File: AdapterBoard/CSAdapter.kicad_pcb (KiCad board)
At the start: 2 copper layers, 10.4 x 18 mm, 3 parts, among them J1 Conn_01x04, J2 Conn_01x06, SW1 CHS-01

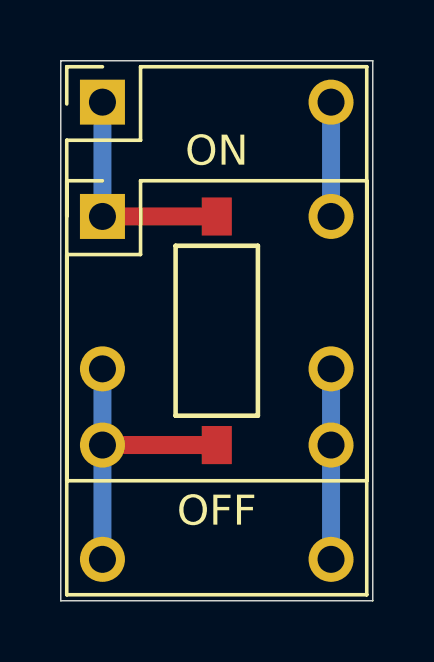
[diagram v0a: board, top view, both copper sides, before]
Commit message: Design rules and gerber files
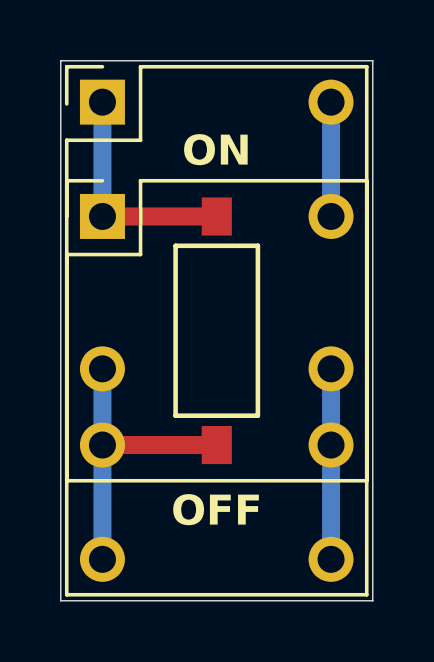
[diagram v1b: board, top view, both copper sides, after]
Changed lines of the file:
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@@
 	)
 	(setup
+		(stackup
+			(layer "F.SilkS"
+				(type "Top Silk Screen")
+			)
+			(layer "F.Paste"
+				(type "Top Solder Paste")
+			)
+			(layer "F.Mask"
+				(type "Top Solder Mask")
+				(thickness 0.01)
+			)
+			(layer "F.Cu"
+				(type "copper")
+				(thickness 0.035)
+			)
+			(layer "dielectric 1"
+				(type "core")
+				(thickness 1.51)
+				(material "FR4")
+				(epsilon_r 4.5)
+				(loss_tangent 0.02)
+			)
+			(layer "B.Cu"
+				(type "copper")
+				(thickness 0.035)
+			)
+			(layer "B.Mask"
+				(type "Bottom Solder Mask")
+				(thickness 0.01)
+			)
+			(layer "B.Paste"
+				(type "Bottom Solder Paste")
+			)
+			(layer "B.SilkS"
+				(type "Bottom Silk Screen")
+			)
+			(copper_finish "None")
+			(dielectric_constraints no)
+		)
 		(pad_to_mask_clearance 0)
 		(allow_soldermask_bridges_in_footprints no)
@@
 			(plot_on_all_layers_selection 0x0000000_00000000)
 			(disableapertmacros no)
-			(usegerberextensions no)
+			(usegerberextensions yes)
 			(usegerberattributes yes)
 			(usegerberadvancedattributes yes)
-			(creategerberjobfile yes)
+			(creategerberjobfile no)
 			(dashed_line_dash_ratio 12.000000)
 			(dashed_line_gap_ratio 3.000000)
@@
 			(psa4output no)
 			(plotreference yes)
-			(plotvalue yes)
+			(plotvalue no)
 			(plotfptext yes)
 			(plotinvisibletext no)
 			(sketchpadsonfab no)
-			(subtractmaskfromsilk no)
+			(subtractmaskfromsilk yes)
 			(outputformat 1)
 			(mirror no)
-			(drillshape 1)
+			(drillshape 0)
 			(scaleselection 1)
-			(outputdirectory "")
+			(outputdirectory "Gerber/")
 		)
 	)
@@
 				(font
 					(size 1 1)
-					(thickness 0.15)
+					(thickness 0.2)
+					(bold yes)
 				)
 			)
@@
 				(font
 					(size 1 1)
-					(thickness 0.15)
-				)
-			)
+					(thickness 0.2)
+					(bold yes)
+				)
+			)
